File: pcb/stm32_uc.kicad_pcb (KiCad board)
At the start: 2 copper layers, 28 parts, among them J1 Conn_01x18_Male, J2 Conn_01x18_Male, J3 USB_C_Receptacle_USB2.0, J4 Conn_01x04_Male, SW1 SW_SPDT, U1 AMS1117-3.3, U2 STM32F103C8T6, Y1 16Mhz

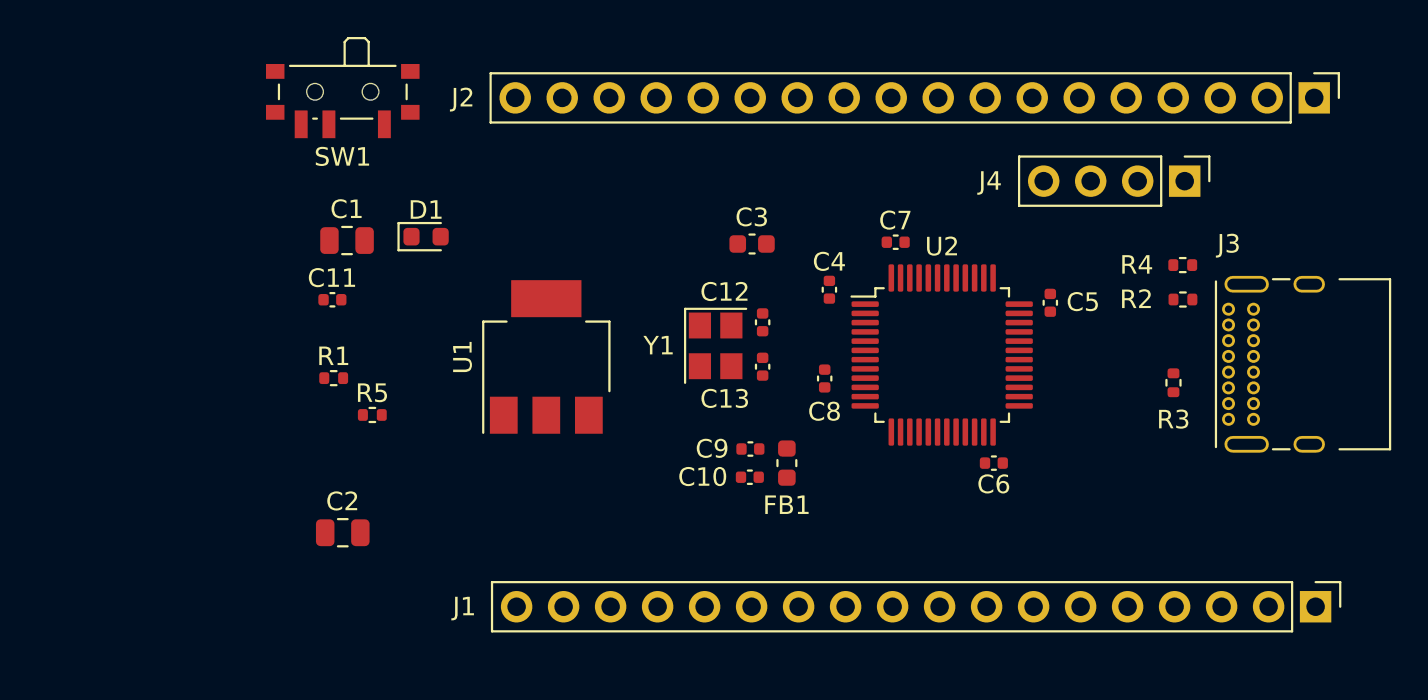
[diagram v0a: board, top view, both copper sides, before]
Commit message: finished rough layout
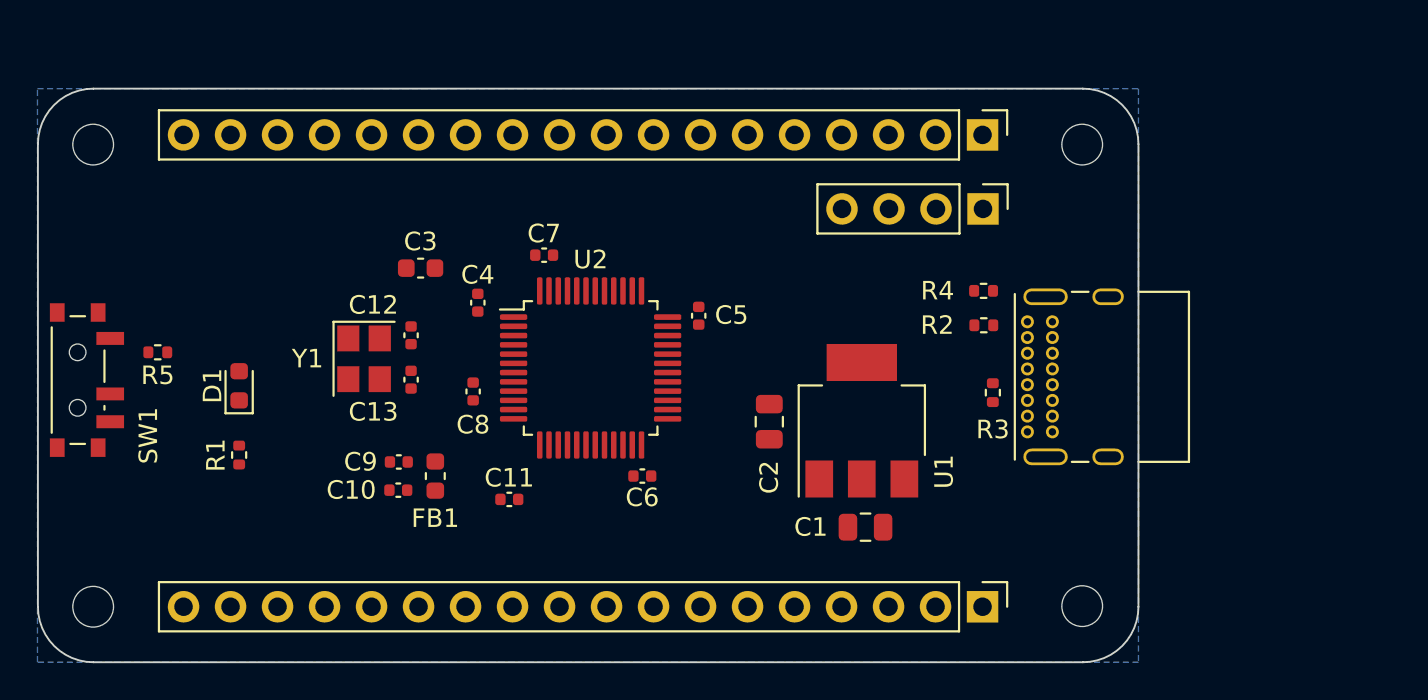
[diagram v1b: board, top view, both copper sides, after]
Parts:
- added H1: MountingHole, MountingHole:MountingHole_2.2mm_M2, F.Cu at (188.0, 117.0)
- added H2: MountingHole, MountingHole:MountingHole_2.2mm_M2, F.Cu at (134.5, 92.0)
- added H3: MountingHole, MountingHole:MountingHole_2.2mm_M2, F.Cu at (134.5, 117.0)
- added H4: MountingHole, MountingHole:MountingHole_2.2mm_M2, F.Cu at (188.0, 92.0)
- moved C1 32.0 mm to (176.2, 112.7), turned to 180 degrees
- moved C2 23.8 mm to (171.1, 107.0), turned to -90 degrees
- moved SW1 20.7 mm to (134.0, 104.8), turned to -90 degrees
- moved C10 19.0 mm to (151.0, 110.7)
- moved C12 19.0 mm to (151.7, 102.3)
- moved C13 19.0 mm to (151.7, 104.7)
- moved C4 19.0 mm to (155.3, 100.6)
- moved C5 19.0 mm to (167.2, 101.3)
- moved C6 19.0 mm to (164.2, 109.9)
- moved C7 19.0 mm to (158.9, 98.0)
- moved C8 19.0 mm to (155.0, 105.4)
- moved C9 19.0 mm to (151.0, 109.2)
- moved FB1 19.0 mm to (153.0, 109.9)
- moved U2 19.0 mm to (161.4, 104.1)
- moved Y1 19.0 mm to (149.2, 103.6)
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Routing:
- added copper zone on B.Cu, net GND
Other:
- board outline added: 59.5 x 31 mm
